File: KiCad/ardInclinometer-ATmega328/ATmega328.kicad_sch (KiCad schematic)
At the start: 14 parts, among them J1 Power in, J2 FTDI, U3 AMS1117-5.0, U4 ATmega328P-PU, Y1 16MHz

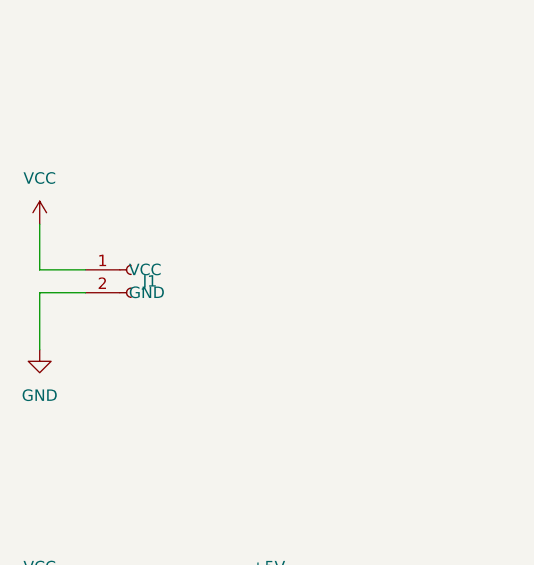
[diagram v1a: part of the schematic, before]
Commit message: kicad7
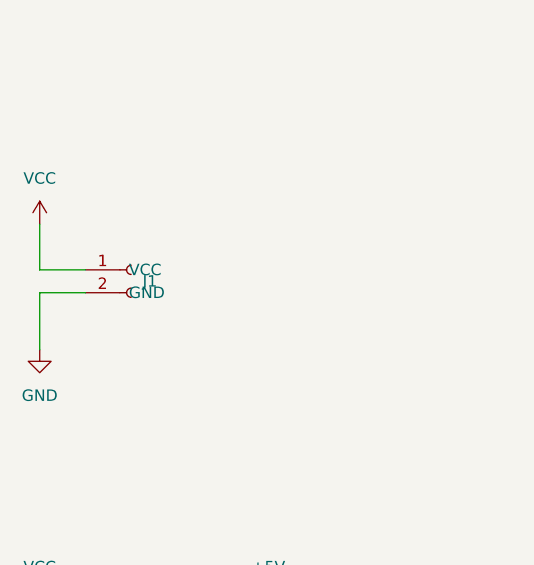
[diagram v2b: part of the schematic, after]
